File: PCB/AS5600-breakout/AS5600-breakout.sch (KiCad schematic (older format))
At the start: 1 part, among them U1 AS5600

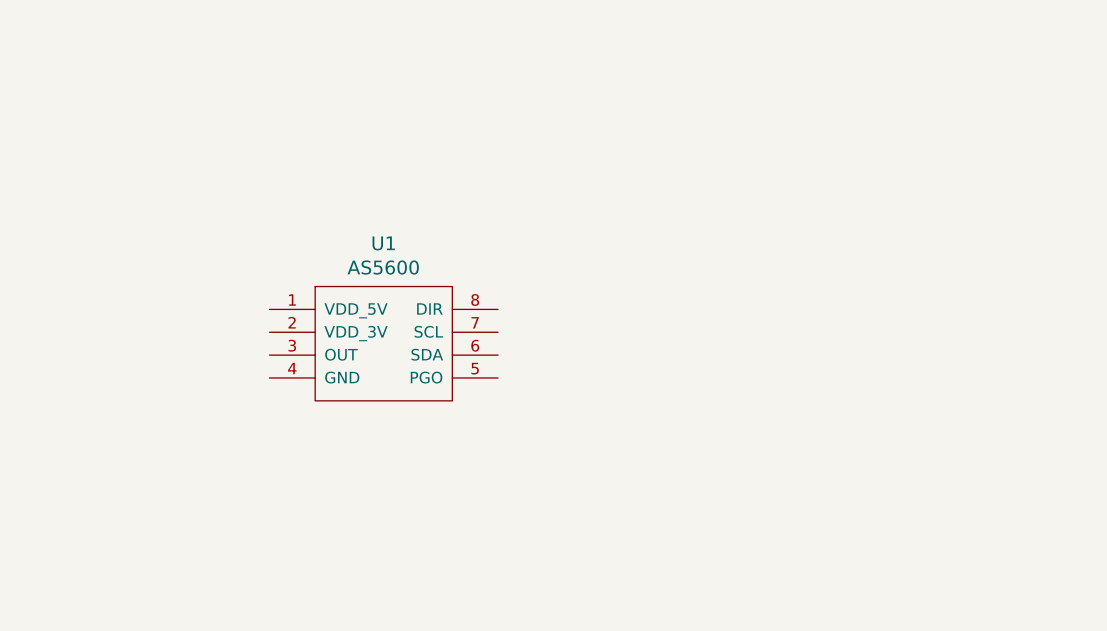
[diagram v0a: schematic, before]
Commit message: initial PCB for encoder
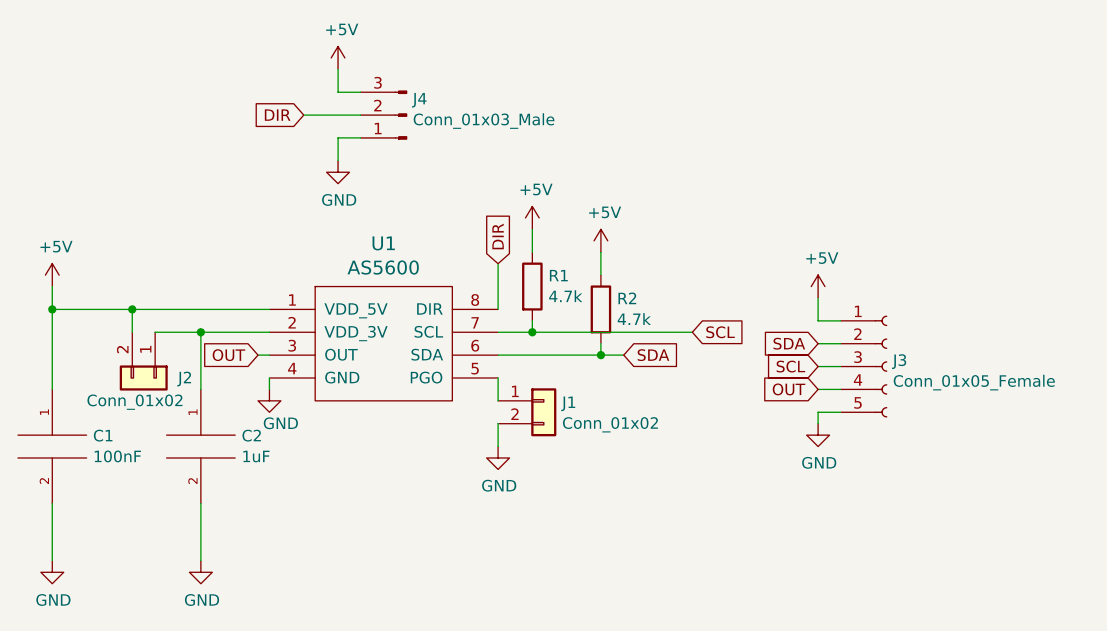
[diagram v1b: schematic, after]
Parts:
- added C1: 100nF, Capacitor_THT:CP_Radial_D6.3mm_P2.50mm, symbol pspice:CAP
- added C2: 1uF, Capacitor_THT:CP_Radial_D8.0mm_P3.50mm, symbol pspice:CAP
- added J1, J2: Conn_01x02, Connector_PinHeader_2.54mm:PinHeader_1x02_P2.54mm_Vertical, symbol Connector_Generic:Conn_01x02
- added J3: Conn_01x05_Female, Connector_PinHeader_2.54mm:PinHeader_1x05_P2.54mm_Horizontal, symbol Connector:Conn_01x05_Female
- added J4: Conn_01x03_Male, Connector_PinHeader_2.54mm:PinHeader_1x03_P2.54mm_Vertical, symbol Connector:Conn_01x03_Male
- added R1, R2: 4.7k, Resistor_THT:R_Axial_DIN0207_L6.3mm_D2.5mm_P7.62mm_Horizontal, symbol Device:R
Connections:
- net +5V: now reaches U1.1 (VDD_5V)
- net +5V: now also C1.1, J2.2 (Pin_2), J3.1 (Pin_1), J4.3 (Pin_3), R1.1, R2.1
- net at U1.2 (VDD_3V): now also C2.1, J2.1 (Pin_1)
- net OUT: now reaches U1.3 (OUT)
- net OUT: now also J3.4 (Pin_4)
- net GND: now reaches U1.4 (GND)
- net GND: now also C1.2, C2.2, J1.2 (Pin_2), J3.5 (Pin_5), J4.1 (Pin_1)
- net at U1.5 (PGO): now also J1.1 (Pin_1)
- net SDA: now reaches U1.6 (SDA)
- net SDA: now also J3.2 (Pin_2), R2.2
- net SCL: now reaches U1.7 (SCL)
- net SCL: now also J3.3 (Pin_3), R1.2
- net DIR: now reaches U1.8 (DIR)
- net DIR: now also J4.2 (Pin_2)
